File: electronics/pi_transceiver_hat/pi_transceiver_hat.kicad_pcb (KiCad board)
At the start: 4 copper layers, 65 x 56 mm, 40 parts, among them J1 Raspberry_Pi_2_3, J10 +5v Power, J11 i2c, J12 i2c, J13 i2c, J14 i2c, J15 Meter, J2 GND, J3 RX Board, J4 1 wire, J5 PSU Board, J6 +5V, J7 UART, J8 +3.3V, J9 PA Board, M1 Fan 1, M2 Fan 2, Q1 2N7000, Q2 2N7000, U1 MCP4725xxx-xCH

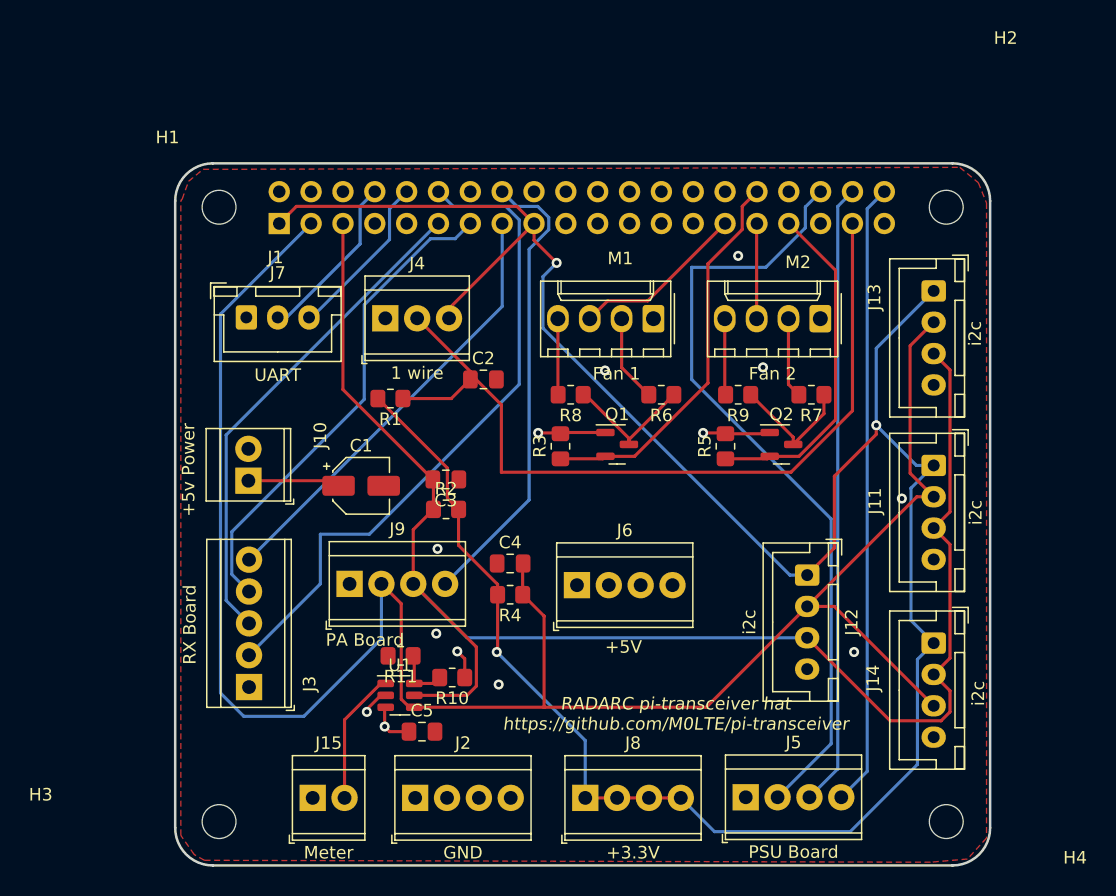
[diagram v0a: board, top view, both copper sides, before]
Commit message: Gerber generation for hat.
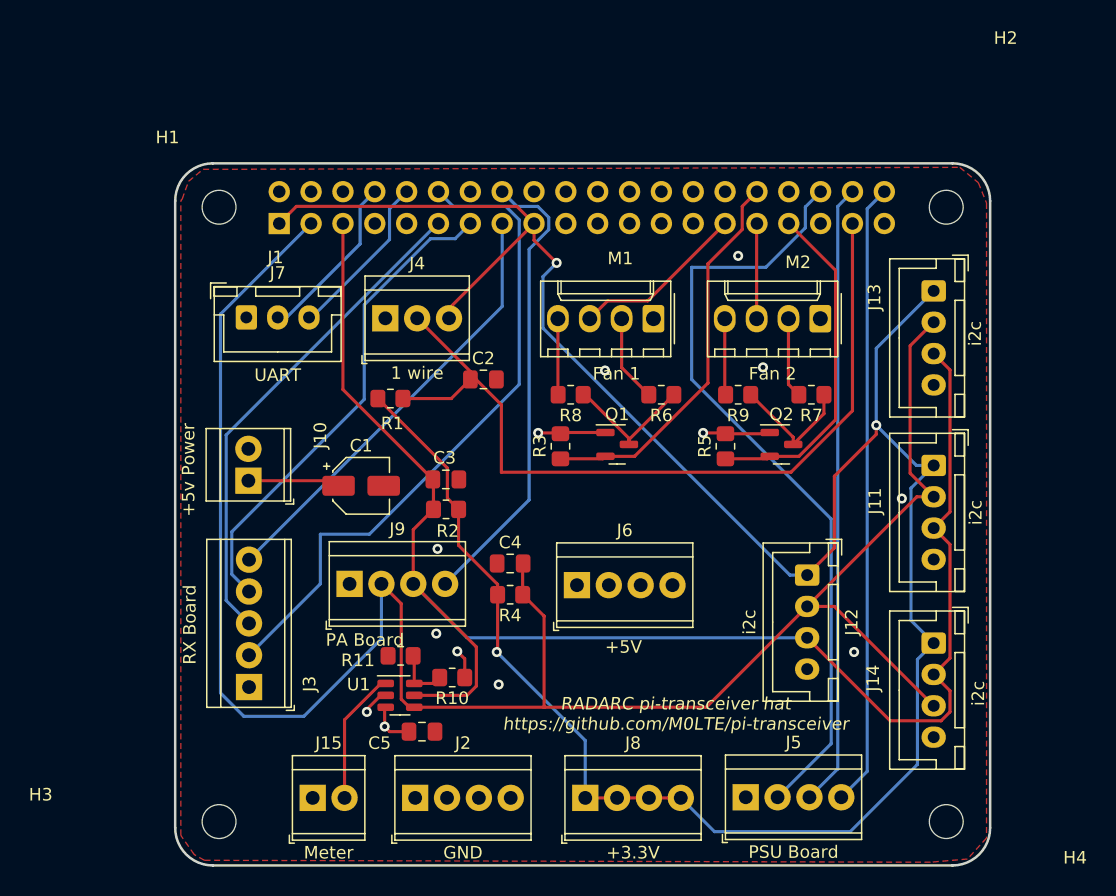
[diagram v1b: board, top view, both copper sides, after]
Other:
- rule pad_to_mask_clearance: 0.051 -> 0
